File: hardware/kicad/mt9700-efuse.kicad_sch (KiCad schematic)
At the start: 9 parts, among them U67 MT9700-N, U68 150uF

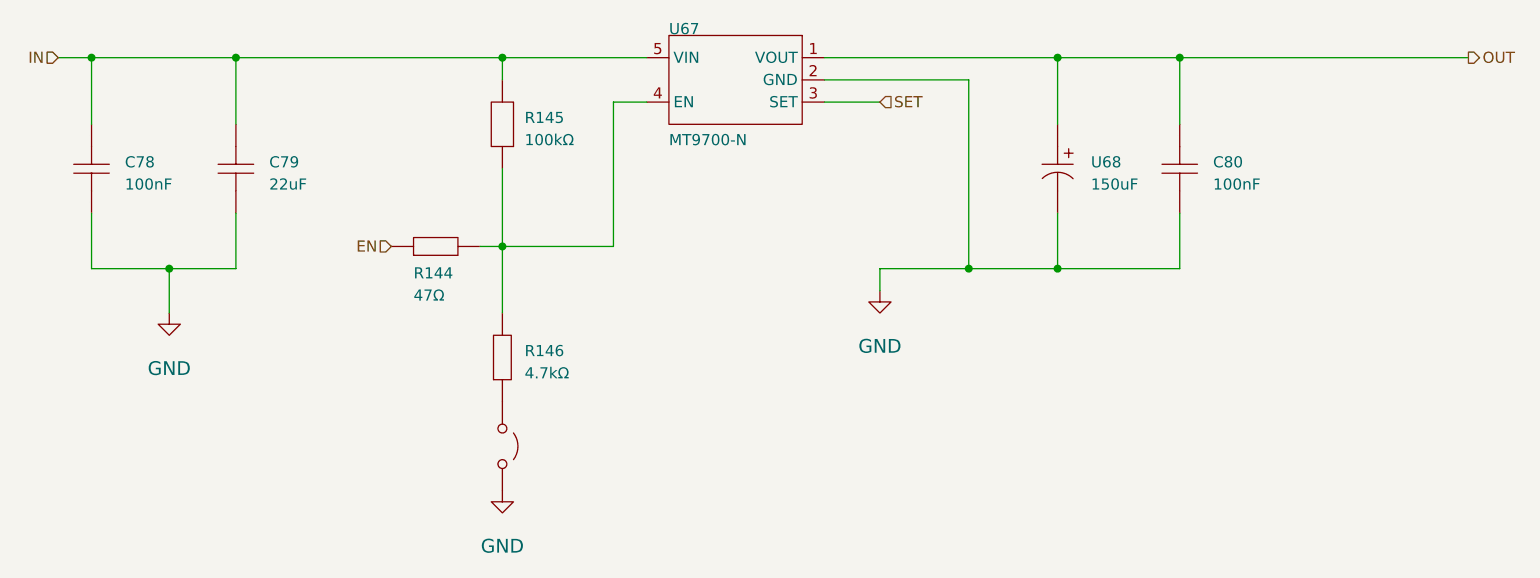
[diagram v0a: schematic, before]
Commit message: various improvements
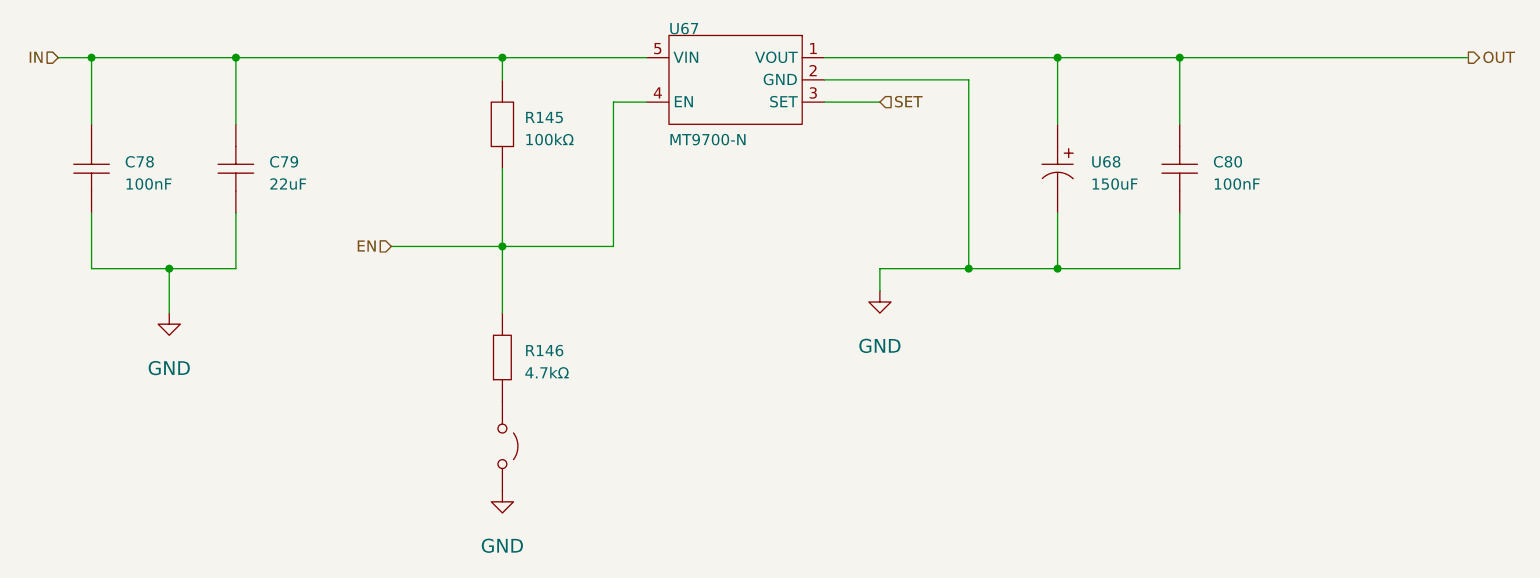
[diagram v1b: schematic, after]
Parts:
- removed R144: 47Ω, 5v rail sm-easyedapro:R0603, symbol 5v rail sm-easyedapro:RS-03K47R0FT
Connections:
- net EN: now also R145.1, R146.2, U67.4 (EN)
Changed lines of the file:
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@@
-	(wire
-		(pts
-			(xy 114.3 97.79) (xy 116.84 97.79)
-		)
-		(stroke
-			(width 0)
-			(type default)
-		)
-	)
 	(wire
 		(pts
@@
 		(pts
 			(xy 129.54 97.79) (xy 129.54 81.28)
+		)
+		(stroke
+			(width 0)
+			(type default)
+		)
+	)
+	(wire
+		(pts
+			(xy 104.14 97.79) (xy 116.84 97.79)
 		)
 		(stroke
@@
 					(unit 1)
 				)
-			)
-		)
-	)
-	(symbol
-		(lib_id "5v rail sm-easyedapro:RS-03K47R0FT")
-		(at 109.22 97.79 0)
-		(unit 1)
-		(exclude_from_sim no)
-		(in_bom yes)
-		(on_board yes)
-		(dnp no)
-		(property "Reference" "R144"
-			(at 106.68 101.6 0)
-			(effects
-				(font
-					(size 1.27 1.27)
-				)
-				(justify left bottom)
-			)
-		)
-		(property "Value" "47Ω"
-			(at 106.68 104.14 0)
-			(effects
-				(font
-					(size 1.27 1.27)
-				)
-				(justify left bottom)
-			)
-		)
-		(property "Footprint" "5v rail sm-easyedapro:R0603"
-			(at 109.22 97.79 0)
-			(effects
-				(font
-					(size 1.27 1.27)
-				)
-				(hide yes)
-			)
-		)
-		(property "Datasheet" "https://atta.szlcsc.com/upload/public/pdf/source/20140616/1457707091974.pdf"
-			(at 109.22 97.79 0)
-			(effects
-				(font
-					(size 1.27 1.27)
-				)
-				(hide yes)
-			)
-		)
-		(property "Description" "Type:Thick Film Resistors Resistance: Tolerance:±1% Tolerance:±1% Power(Watts): Overload Voltage (Max): Temperature Coefficient:±100ppm/°C Temperature Coefficient:±100ppm/°C Operating Temperature Range:-55°C~+155°C Operating Temperature Range:-55°C~+155°C"
-			(at 109.22 97.79 0)
-			(effects
-				(font
-					(size 1.27 1.27)
-				)
-				(hide yes)
-			)
-		)
-		(property "Manufacturer Part" "RS-03K47R0FT"
-			(at 109.22 97.79 0)
-			(effects
-				(font
-					(size 1.27 1.27)
-				)
-				(hide yes)
-			)
-		)
-		(property "Manufacturer" "FH(风华)"
-			(at 109.22 97.79 0)
-			(effects
-				(font
-					(size 1.27 1.27)
-				)
-				(hide yes)
-			)
-		)
-		(property "Supplier Part" "C140087"
-			(at 109.22 97.79 0)
-			(effects
-				(font
-					(size 1.27 1.27)
-				)
-				(hide yes)
-			)
-		)
-		(property "Supplier" "LCSC"
-			(at 109.22 97.79 0)
-			(effects
-				(font
-					(size 1.27 1.27)
-				)
-				(hide yes)
-			)
-		)
-		(property "LCSC Part Name" "厚膜电阻 47Ω ±1% 100mW"
-			(at 109.22 97.79 0)
-			(effects
-				(font
-					(size 1.27 1.27)
-				)
-				(hide yes)
-			)
-		)
-		(pin "1"
-		)
-		(pin "2"
-		)
-		(instances
-			(project "svea_powerboard_rev3"
-				(path "/3f85abf4-0b95-4c4a-b7e9-06f59ca1ea3d/5c2e021f-c2d4-49e2-8c36-9a64f1f12001/1d4a251e-4375-4aab-85e0-d11dfb5595c0"
-					(reference "R144")
-					(unit 1)
-				)
-				(path "/3f85abf4-0b95-4c4a-b7e9-06f59ca1ea3d/5c2e021f-c2d4-49e2-8c36-9a64f1f12001/a553934f-48fa-4d71-a435-79ebd566d680"
-					(reference "R167")
-					(unit 1)
-				)
